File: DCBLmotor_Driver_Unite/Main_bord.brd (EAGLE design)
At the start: 160 x 94.5 mm, 54 parts, among them CN1 DF11-16DP-2DSA, CN2 DF11-16DP-2DSA, CN3 DF11-4DP-2DSR, CN4 HIF3FC-10PA-2.54DSA(71), CN5 HIF3FC-10PA-2.54DSA(71), CN6 0430450612, CN7 0430450612, IC1 TMPM370FYFG, IC2 MCP2561FD-E/MF, IC3 AM26C32CD, IC4 AM26C32CD, SW1 CVS-02TB, SW2 EVQ-PE104K

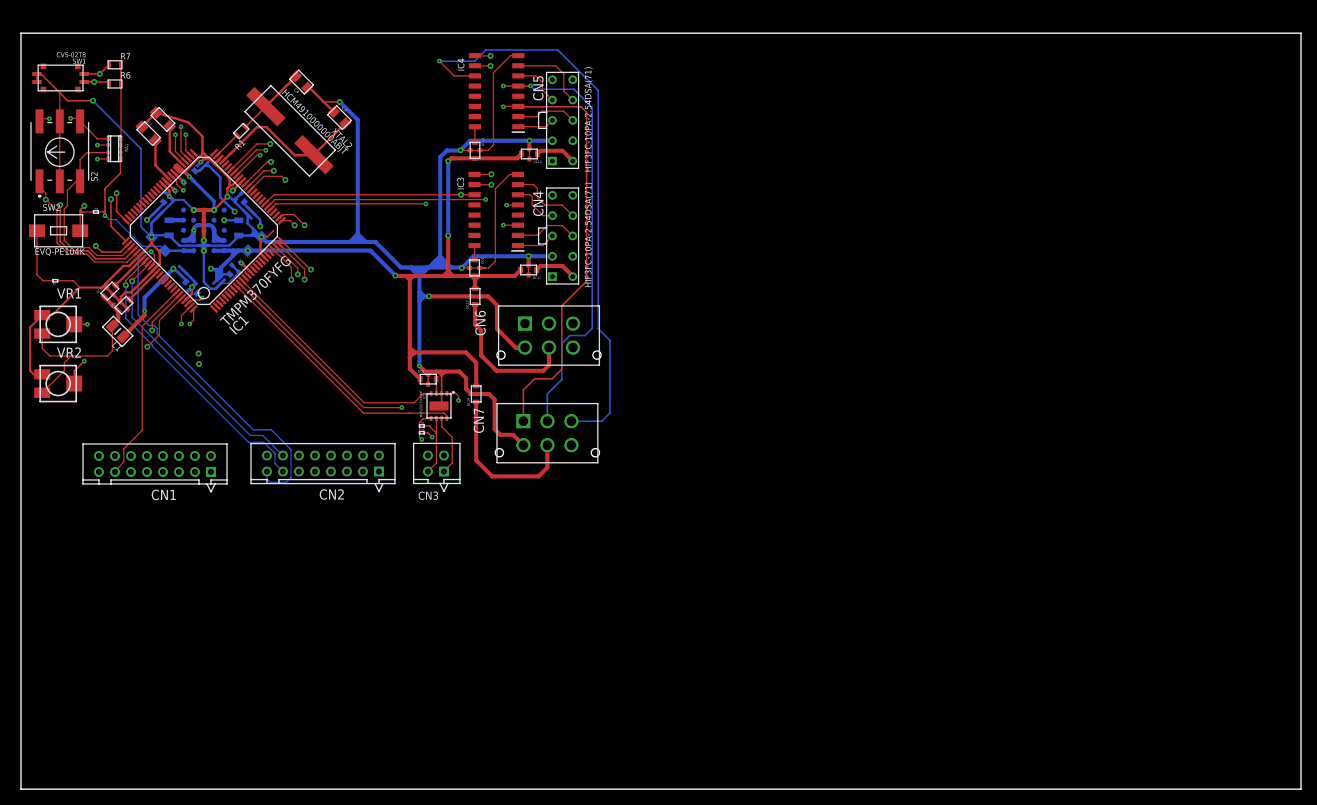
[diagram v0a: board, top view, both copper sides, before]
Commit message: Version1 per finshed
Per complete Version1
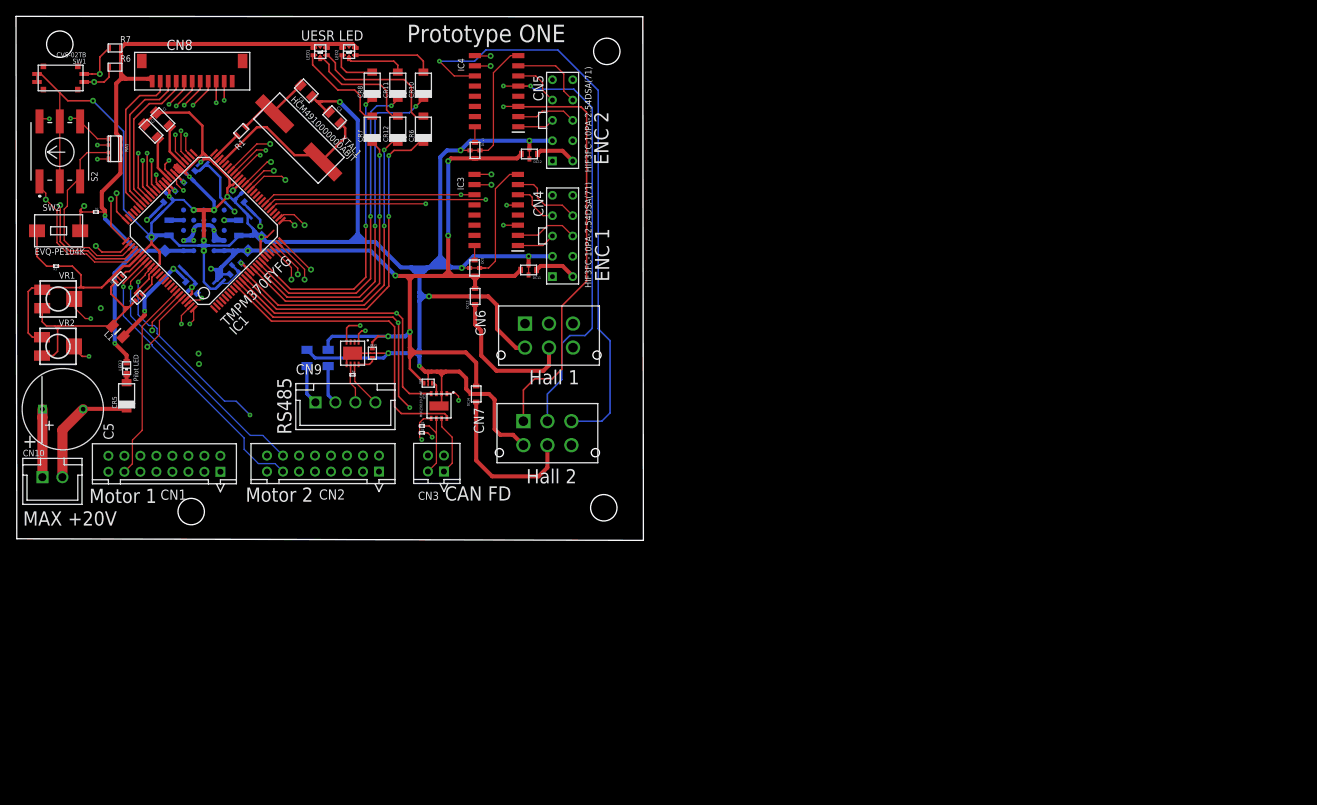
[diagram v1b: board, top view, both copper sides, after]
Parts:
- removed XTAL2: HCM4910000000ABJT, Citizen:HCM49
- added 0R1, 0R2: 5106, Keystone:5106JUMP_0805
- added C5: T356L107K016AT, KEMET:T356
- added CN10: (no value), jst-xh:B2B-XH-A
- added CN8: BM11B-SRSS-TB, JST:BM11B-SRSS-TB
- added CN9: (no value), jst-xh:B4B-XH-A
- added CR10, CR11, CR12, CR5, CR6, CR7, CR8: NSI50010YT1G, ON Semiconductor:SOD-123
- added DC15: YFF15PC1C104MT000N, TDK:YFF15PC
- added IC5: LTC2862A, LT:DD_PACKGE_8
- added LED1, LED2: CL-340T-SD-T, Citizen:CL-340
- added LED3: CL-196YG-CD-T, Citizen:CL-196
- added R8: MCR006, ROHM:MCR006
- added XTAL1: HCM4910000000ABJT, Citizen:HCM49
- DC6, DC7, DC8: value YFF21PC -> YFF15PC1C104MT000N; device TDK:YFF21PC -> TDK:YFF15PC
- moved VR2 4.65 mm to (4.62, 55.4)
- moved VR1 3.17 mm to (4.65, 61.3)
- moved R7 2.10 mm to (12.5, 92.7)
- moved R6 2.10 mm to (12.5, 90.2)
- moved DC6 2.09 mm to (14.7, 61.5)
- moved DC7 1.95 mm to (12.3, 63.8)
- moved R3 1.83 mm to (4.10, 65.4)
- moved C4 1.25 mm to (35.0, 88.0)
- moved CN1 1.18 mm to (24.9, 39.7)
- moved C3 0.60 mm to (39.9, 83.2)
- moved DC8 0.50 mm to (50.9, 50.8)
- moved C2 0.42 mm to (17.1, 81.4)
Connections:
- new net A*: CN9.3, IC5.P$6, R8.P$2
- new net B*: CN9.4, IC5.P$7, R8.P$1
- new net LED1_1: CR6.P$C, IC1.P$12
- new net LED1_2: CR12.P$C, IC1.P$13
- new net LED1_3: CR7.P$C, IC1.P$15
- new net LED2_1: CR10.P$C, IC1.P$16
- new net LED2_2: CR11.P$C, IC1.P$17
- new net LED2_3: CR8.P$C, IC1.P$18
- new net N$34: CR5.P$A, LED3.P$C
- new net N$37: CR7.P$A, LED1.P$4
- new net N$38: CR12.P$A, LED1.P$5
- new net N$39: CR6.P$A, LED1.P$6
- new net N$40: CR8.P$A, LED2.P$4
- new net N$41: CR11.P$A, LED2.P$5
- new net N$42: CR10.P$A, LED2.P$6
- new net N$43: DC15.P$1, IC5.P$8
- new net N$44: 0R2.P$1, CN9.2
- new net N$46: 0R1.P$1, CN9.1
- net +5V: now also 0R2.P$2, DC15.P$2
- net GND: now also 0R1.P$2, C5.P$-, CN10.2, CR5.P$C, DC15.P$3, DC15.P$4, DC6.P$3, DC6.P$4, DC7.P$3, DC7.P$4, DC8.P$3, DC8.P$4, IC5.P$5, IC5.PAD; no longer DC6.GND1, DC6.GND2, DC7.GND1, DC7.GND2, DC8.GND1, DC8.GND2
- net N$11: now also XTAL1.P$2; no longer XTAL2.P$2
- net N$18: now also CN8.P$5
- net N$19: now also CN8.P$6
- net N$20: now also CN8.P$9
- net N$21: now also CN8.P$7
- net N$22: now also CN8.P$8
- net N$23: now also CN8.P$4
- net N$24: now also CN8.P$3
- net N$25: now also CN8.P$2
- net RESET: now also CN8.P$10
- net RX0: now also IC5.P$4
- net TX0: now also IC5.P$1
- net VCC: now also CN8.P$1, LED1.P$1, LED1.P$2, LED1.P$3, LED2.P$1, LED2.P$2, LED2.P$3, LED3.P$A
- net VDD: now also C5.P$+, CN10.1
- net X1: now also XTAL1.P$1; no longer XTAL2.P$1
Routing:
- net GND: track 399.6 -> 471.6 mm, vias 14 -> 16
- net VCC: track 33.8 -> 90.6 mm, vias 1 -> 2
- net LED2_1: track 0.00 -> 44.9 mm, vias 0 -> 2
- net LED1_1: track 0.00 -> 42.1 mm, vias 0 -> 2
- net LED2_2: track 0.00 -> 41.2 mm, vias 0 -> 2
- net LED1_2: track 0.00 -> 38.8 mm, vias 0 -> 2
- net LED2_3: track 0.00 -> 37.7 mm, vias 0 -> 2
- net LED1_3: track 0.00 -> 36.3 mm, vias 0 -> 2
- net N$25: track 0.00 -> 19.4 mm
- net RX0: track 30.4 -> 49.7 mm, vias 0 -> 2
- net N$24: track 0.00 -> 19.0 mm
- net N$23: track 0.00 -> 18.7 mm
- net N$19: track 0.00 -> 17.9 mm, vias 0 -> 2
- net N$39: track 0.00 -> 17.6 mm
- net N$18: track 0.00 -> 17.6 mm, vias 0 -> 2
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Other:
- board size 160 x 94.5 mm -> 78.4 x 65.5 mm
- board text added: "+"
- board text added: "CAN FD"
- board text added: "ENC 1"
- board text added: "ENC 2"
- board text added: "Hall 1"
- board text added: "Hall 2"
- board text added: "MAX +20V"
- board text added: "Motor 1"
- board text added: "Motor 2"
- board text added: "Pilot LED"
- board text added: "Prototype ONE"
- board text added: "RS485"
- board text added: "RS485 Power jumper"
- board text added: "UESR LED"
